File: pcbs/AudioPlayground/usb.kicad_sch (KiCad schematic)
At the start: 19 parts, among them J3 USB_C_Receptacle_USB2.0_14P, U15 USBLC6-2P6, U3 USB2422/MJ, Y3 24MHz

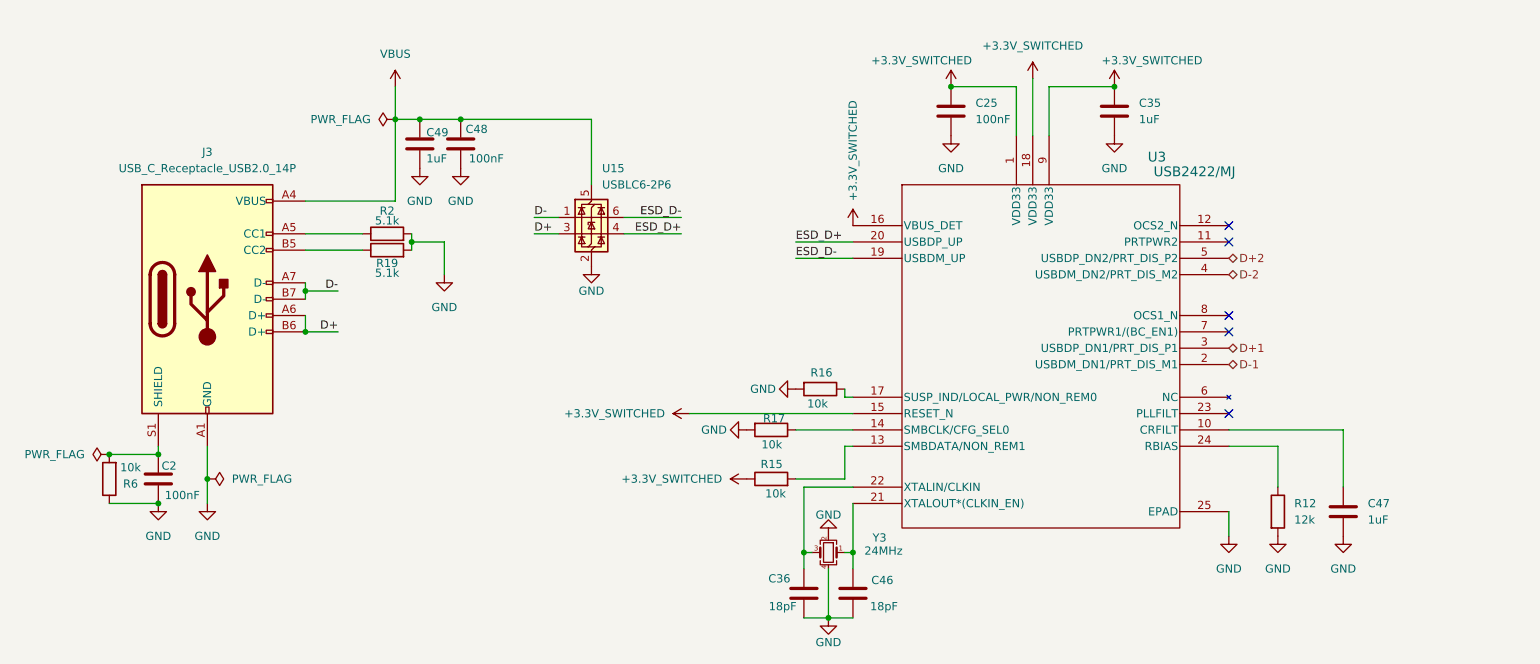
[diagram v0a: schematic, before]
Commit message: Improve Optic
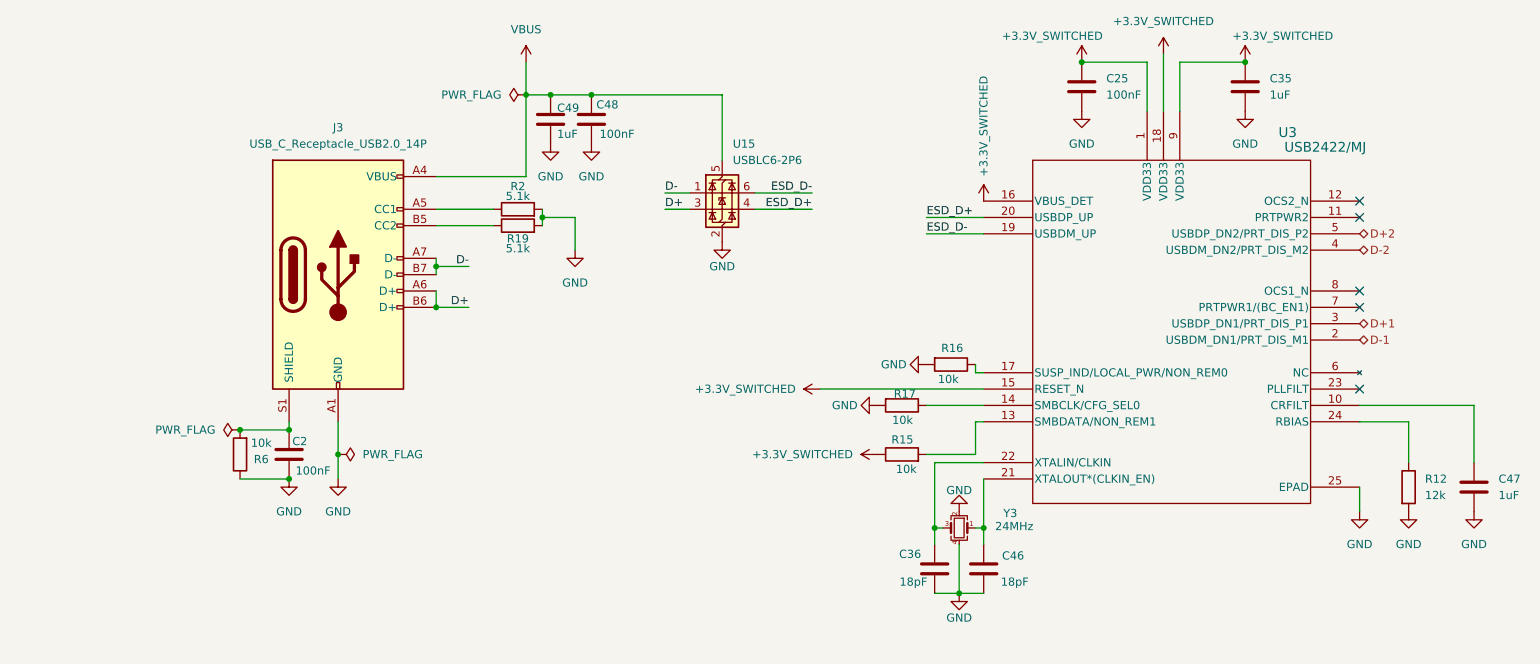
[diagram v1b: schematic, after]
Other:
- title: (none) -> LE Audio Playground
- moved on the sheet: C2, C25, C35, C36, C46, C47, C48, C49, J3, R12, R15, R16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
